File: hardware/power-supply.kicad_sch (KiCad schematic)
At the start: 17 parts, among them U3 LM5164DDA, U4 TPS70933

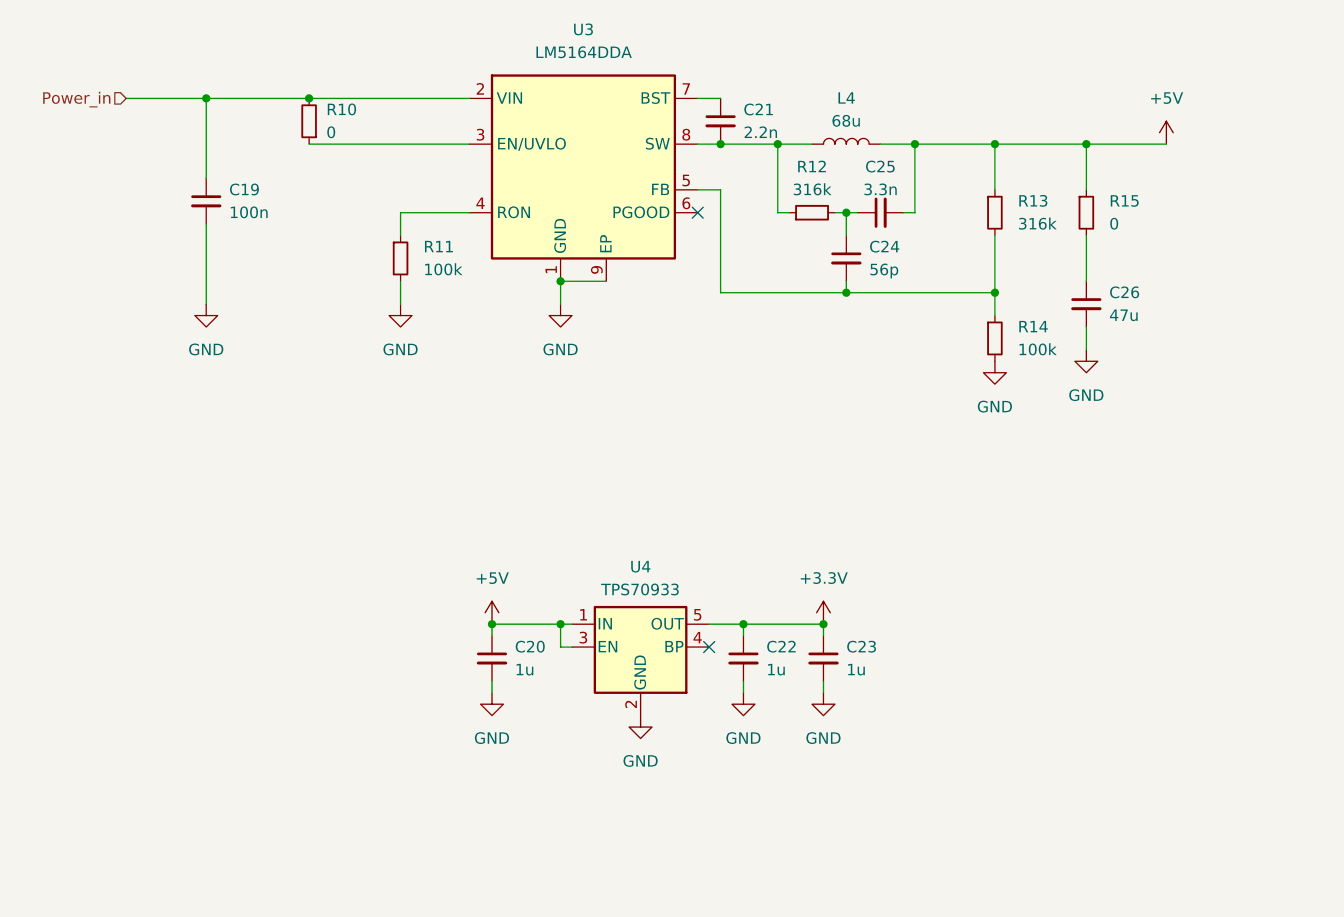
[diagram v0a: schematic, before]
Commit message: Prettyfy Schematic
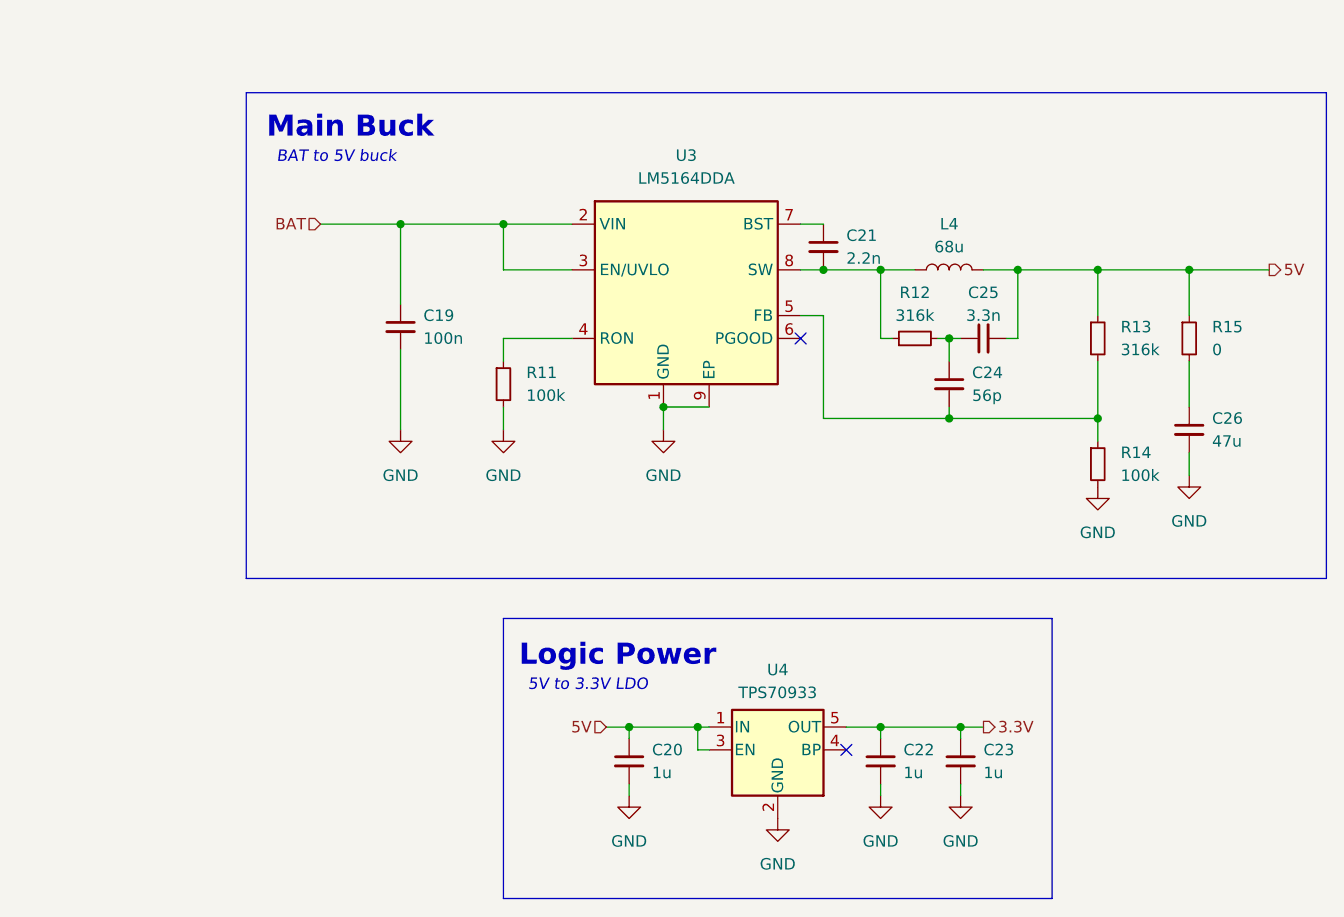
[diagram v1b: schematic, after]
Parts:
- removed R10: 0, Resistor_SMD:R_0402_1005Metric, symbol Device:R_Small
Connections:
- net Power_in is gone; now on net BAT: C19.1, U3.2 (VIN)
- net BAT: now reaches U3.3 (EN/UVLO)
- net +3.3V renamed 3.3V
- net +5V renamed 5V
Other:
- note added: "5V to 3.3V LDO"
- note added: "BAT to 5V buck"
- note added: "Logic Power"
- note added: "Main Buck"
- moved on the sheet: C19, C20, C21, C22, C23, C24, C25, C26, L4, R11, R12, R13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
